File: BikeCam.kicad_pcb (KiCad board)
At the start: 4 copper layers, 26.4 x 16.3 mm, 24 parts, among them J1 USB_OTG, J2 Conn_01x02_Female, J3 Conn_01x02_Male, Q1 IRLZ34N, Q2 IRLZ34N, Q3 IRLML5203, Q4 IRLML5203, SW1 SW_DIP_x01, U1 MCP73831-2-OT, U2 AP9101CK6, U3 MCP1700-3302E_SOT23

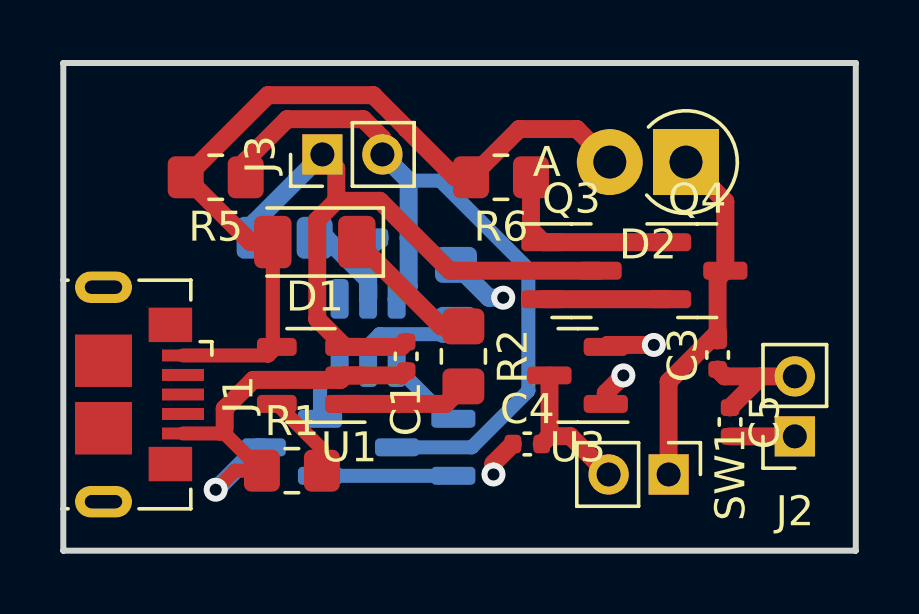
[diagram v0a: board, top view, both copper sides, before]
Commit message: error debug
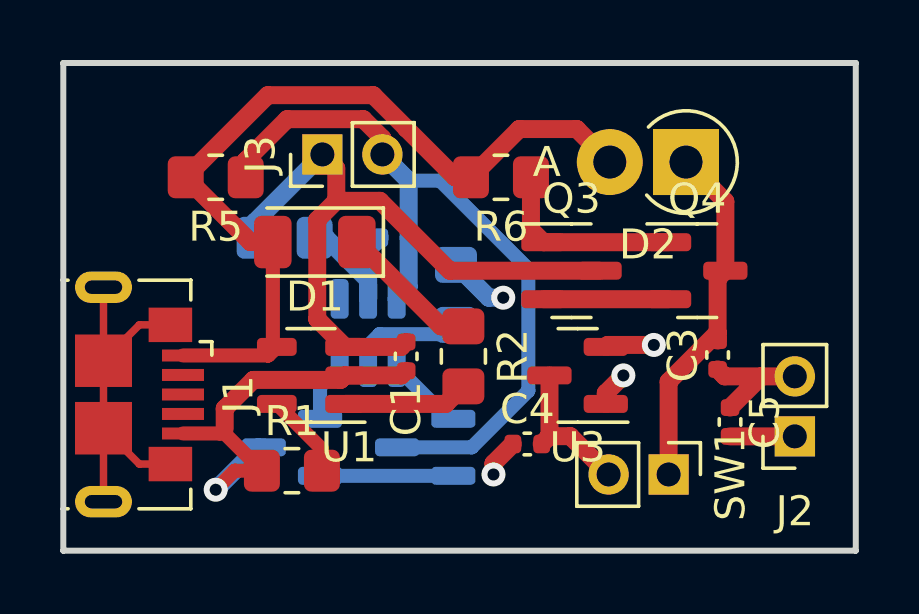
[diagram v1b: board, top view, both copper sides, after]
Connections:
- net +3.3V renamed +3V3
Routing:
- net unconnected-(J1-Pad6): track 0.00 -> 12.6 mm
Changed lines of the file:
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@@
   (net 4 "Net-(C2-Pad2)")
   (net 5 "OUT+")
-  (net 6 "+3.3V")
+  (net 6 "+3V3")
   (net 7 "Net-(D1-Pad1)")
   (net 8 "+5V")
@@
       (net 1 "0V") (pinfunction "GND") (pintype "power_in"))
     (pad "2" smd roundrect (at -0.9375 0.95 180) (size 1.475 0.6) (layers "F.Cu" "F.Paste" "F.Mask") (roundrect_rratio 0.25)
-      (net 6 "+3.3V") (pinfunction "VO") (pintype "power_out"))
+      (net 6 "+3V3") (pinfunction "VO") (pintype "power_out"))
     (pad "3" smd roundrect (at 0.9375 0 180) (size 1.475 0.6) (layers "F.Cu" "F.Paste" "F.Mask") (roundrect_rratio 0.25)
       (net 5 "OUT+") (pinfunction "VI") (pintype "power_in"))
@@
       (net 1 "0V") (pintype "passive"))
     (pad "2" smd roundrect (at 0.48 0 270) (size 0.56 0.62) (layers "F.Cu" "F.Paste" "F.Mask") (roundrect_rratio 0.25)
-      (net 6 "+3.3V") (pintype "passive"))
+      (net 6 "+3V3") (pintype "passive"))
     (model "${KICAD6_3DMODEL_DIR}/Capacitor_SMD.3dshapes/C_0402_1005Metric.wrl"
       (offset (xyz 0 0 0))
@@
     (fp_line (start -1 -1) (end 0.5 -1) (layer "F.Fab") (width 0.1))
     (pad "1" thru_hole rect (at 0 0 180) (size 1.35 1.35) (drill 0.8) (layers *.Cu *.Mask)
-      (net 6 "+3.3V") (pinfunction "Pin_1") (pintype "passive"))
+      (net 6 "+3V3") (pinfunction "Pin_1") (pintype "passive"))
     (pad "2" thru_hole oval (at 0 2 180) (size 1.35 1.35) (drill 0.8) (layers *.Cu *.Mask)
       (net 1 "0V") (pinfunction "Pin_2") (pintype "passive"))
@@
   (segment (start 108.048767 81.450001) (end 106.128999 81.450001) (width 0.6) (layer "F.Cu") (net 8))
   (segment (start 102.368 81.434299) (end 103.991701 83.058) (width 0.6) (layer "F.Cu") (net 8))
+  (segment (start 92.272 91.422) (end 93.467 92.617) (width 0.25) (layer "F.Cu") (net 12))
+  (segment (start 93.467 87.977) (end 94.502 87.977) (width 0.25) (layer "F.Cu") (net 12))
+  (segment (start 92.272 86.722) (end 92.272 89.172) (width 0.25) (layer "F.Cu") (net 12))
+  (segment (start 92.272 91.422) (end 92.272 93.872) (width 0.25) (layer "F.Cu") (net 12))
+  (segment (start 93.467 92.617) (end 94.502 92.617) (width 0.25) (layer "F.Cu") (net 12))
+  (segment (start 92.272 89.172) (end 93.467 87.977) (width 0.25) (layer "F.Cu") (net 12))
+  (segment (start 92.272 89.172) (end 92.272 91.422) (width 0.25) (layer "F.Cu") (net 12))
   (segment (start 99.4895 93.00825) (end 103.9345 93.00825) (width 0.47) (layer "B.Cu") (net 13))
   (segment (start 106.521 84.809) (end 106.934 85.222) (width 0.6) (layer "F.Cu") (net 14))
@@
     )
   )
-  (zone (net 6) (net_name "+3.3V") (layer "In2.Cu") (name "+3.3V") (hatch edge 0.508)
+  (zone (net 6) (net_name "+3V3") (layer "In2.Cu") (name "+3.3V") (hatch edge 0.508)
     (connect_pads (clearance 0.508))
     (min_thickness 0.254) (filled_areas_thickness no)
